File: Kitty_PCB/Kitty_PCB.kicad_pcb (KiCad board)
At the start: 2 copper layers, 90.8 x 99.8 mm, 3 parts, among them J3 Conn_01x06

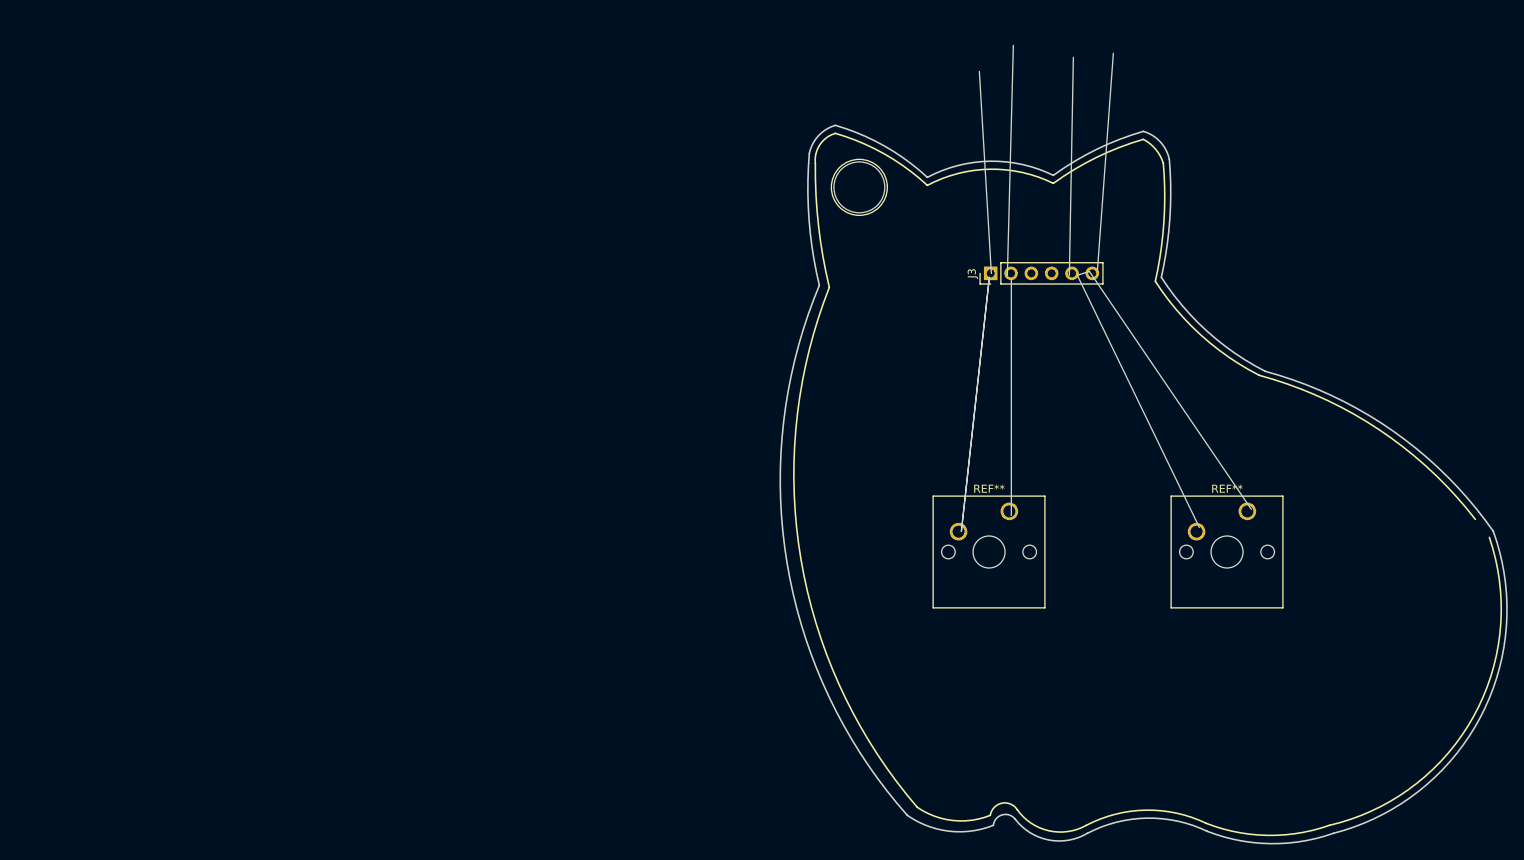
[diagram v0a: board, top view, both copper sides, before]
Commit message: push
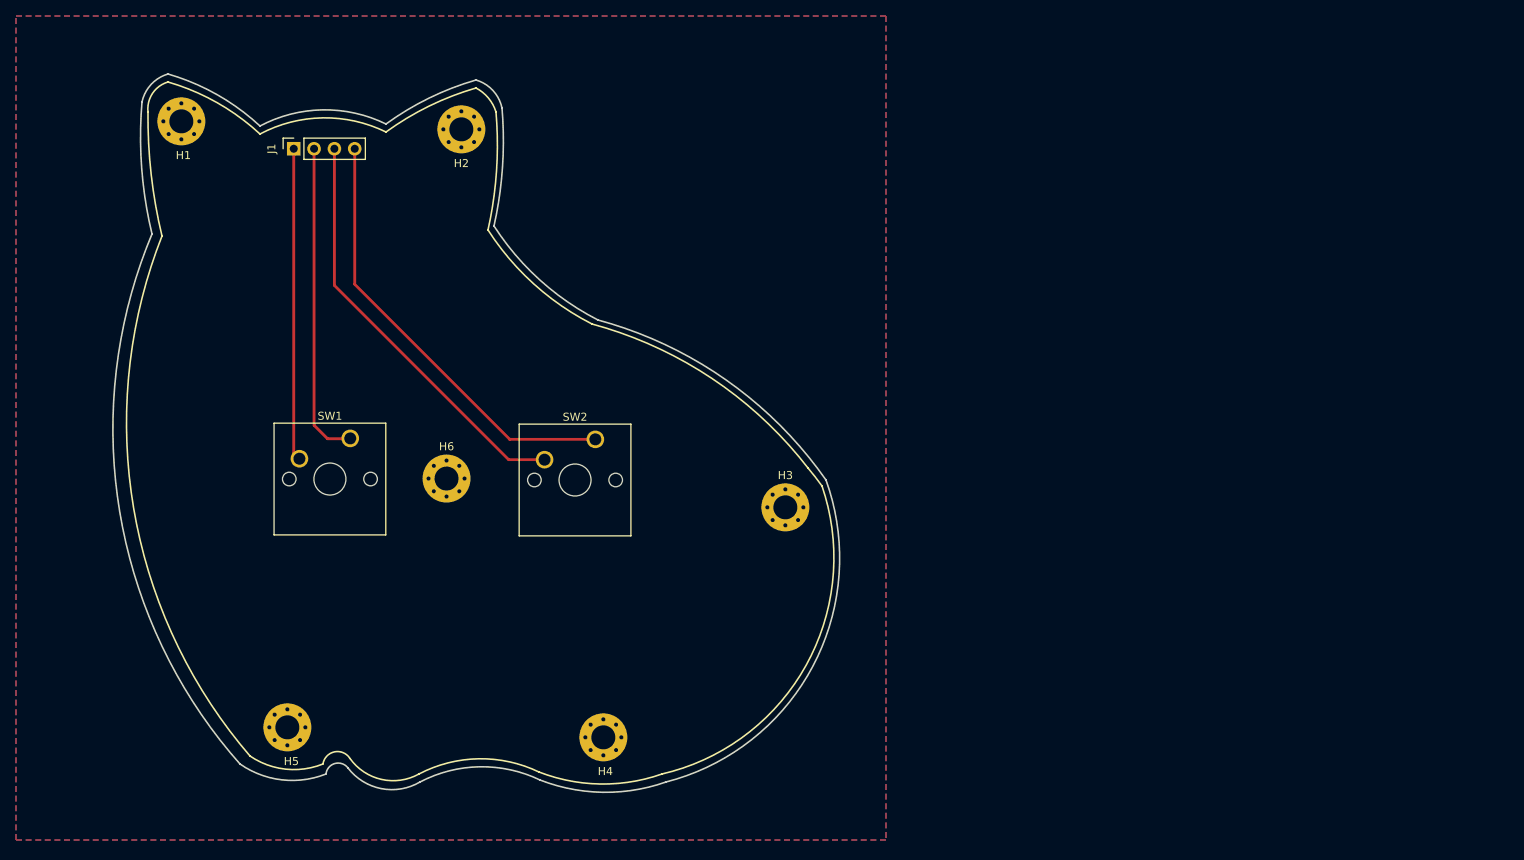
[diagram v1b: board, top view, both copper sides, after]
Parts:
- removed J3: Conn_01x06, Connector_PinHeader_2.54mm:PinHeader_1x06_P2.54mm_Vertical
- removed REF** (x2): SW_Cherry_MX_1.00u_PCB, Button_Switch_Keyboard:SW_Cherry_MX_1.00u_PCB
- added H1: MountingHole_Pad, MountingHole:MountingHole_3mm_Pad_Via, F.Cu at (111.2, 56.2)
- added H2: MountingHole_Pad, MountingHole:MountingHole_3mm_Pad_Via, F.Cu at (146.2, 57.2)
- added H3: MountingHole_Pad, MountingHole:MountingHole_3mm_Pad_Via, F.Cu at (186.8, 104.5)
- added H4: MountingHole_Pad, MountingHole:MountingHole_3mm_Pad_Via, F.Cu at (164.0, 133.2)
- added H5: MountingHole_Pad, MountingHole:MountingHole_3mm_Pad_Via, F.Cu at (124.5, 132.0)
- added H6: MountingHole_Pad, MountingHole:MountingHole_3mm_Pad_Via, F.Cu at (144.4, 100.9)
- added J1: Conn_01x04, Connector_PinSocket_2.54mm:PinSocket_1x04_P2.54mm_Vertical, F.Cu at (125.3, 59.7)
- added SW1: SW_Push, Button_Switch_Keyboard:SW_Cherry_MX_1.00u_PCB, F.Cu at (132.4, 95.9)
- added SW2: SW_Push, Button_Switch_Keyboard:SW_Cherry_MX_1.00u_PCB, F.Cu at (163.0, 96.0)
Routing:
- net Net-(J1-Pad4): track 0.00 -> 55.1 mm
- net Net-(J1-Pad3): track 0.00 -> 52.4 mm
- net Net-(J1-Pad2): track 0.00 -> 39.8 mm
- net Net-(J1-Pad1): track 0.00 -> 39.0 mm
- added copper zone on B.Cu, net GND
- added copper zone on F.Cu, net GND
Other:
- board size 90.8 x 99.8 mm -> 90.8 x 89.8 mm
